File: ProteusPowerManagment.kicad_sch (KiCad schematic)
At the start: 0 parts

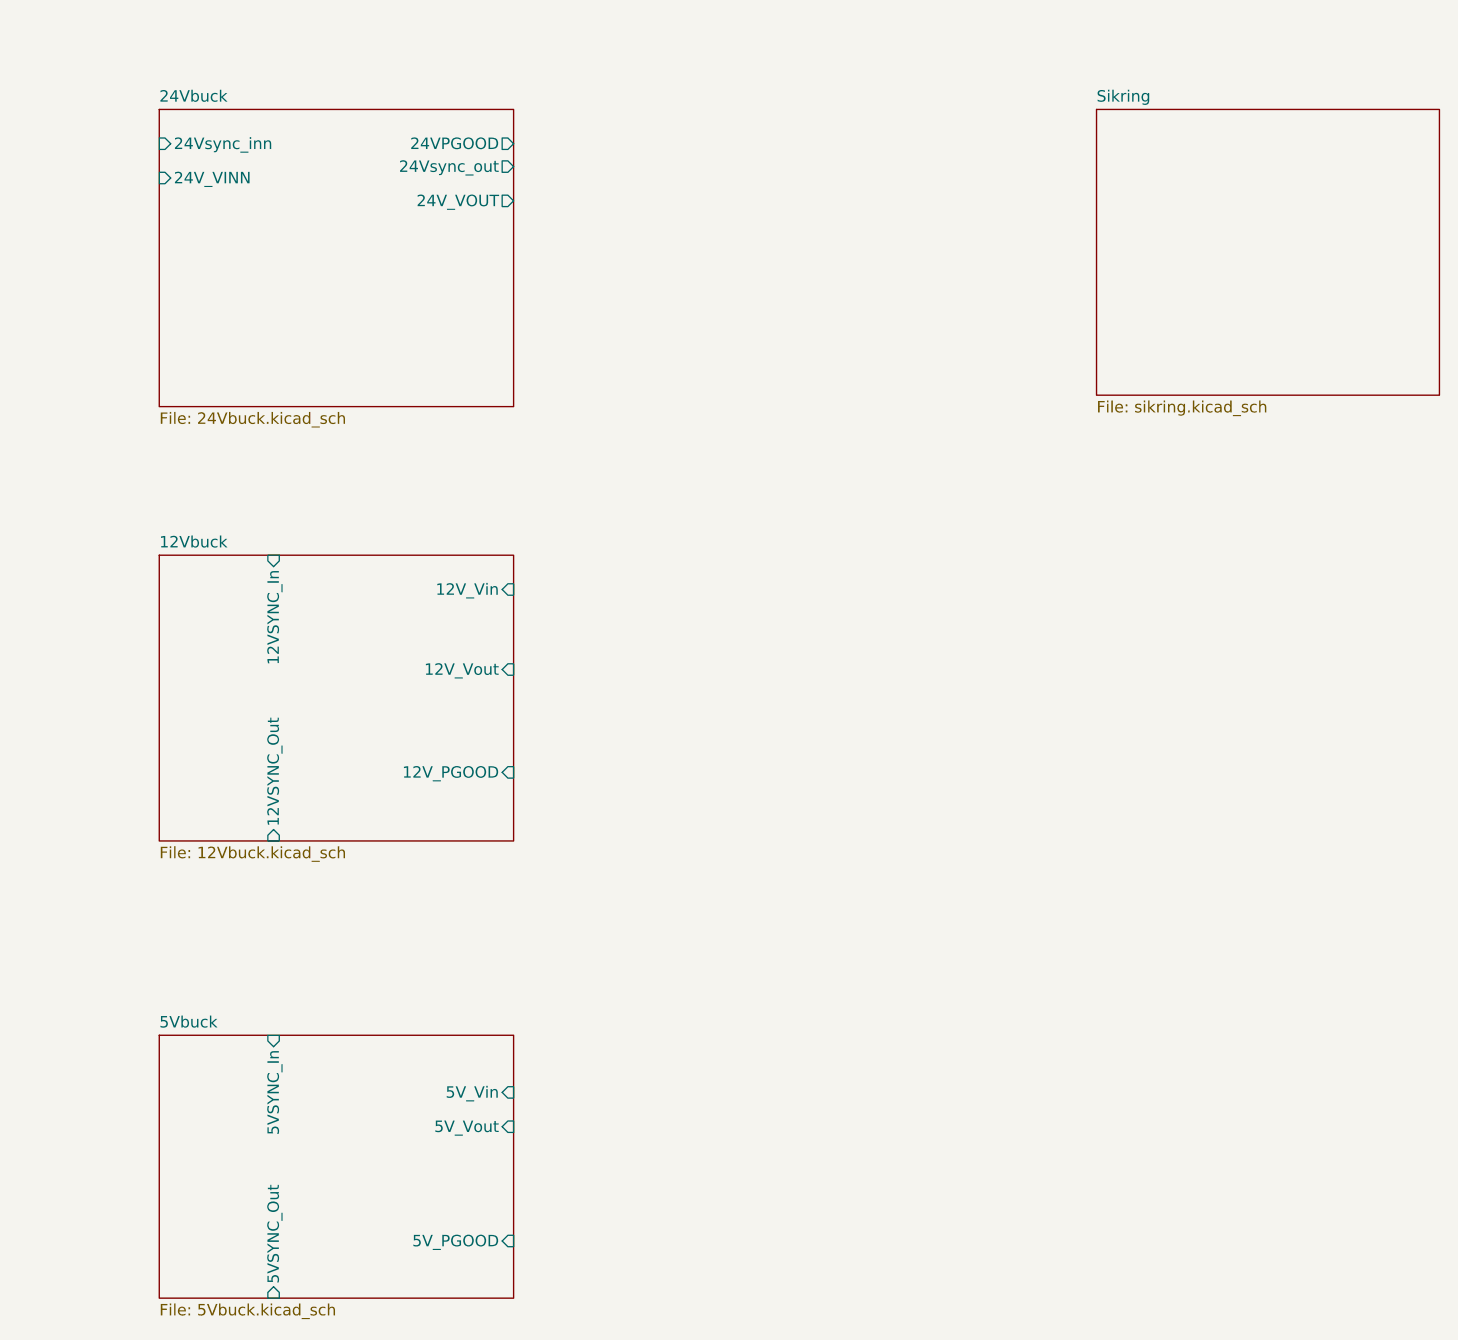
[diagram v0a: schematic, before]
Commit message: lagt inn alle ideele komp mangler å finne faktiske komponenter
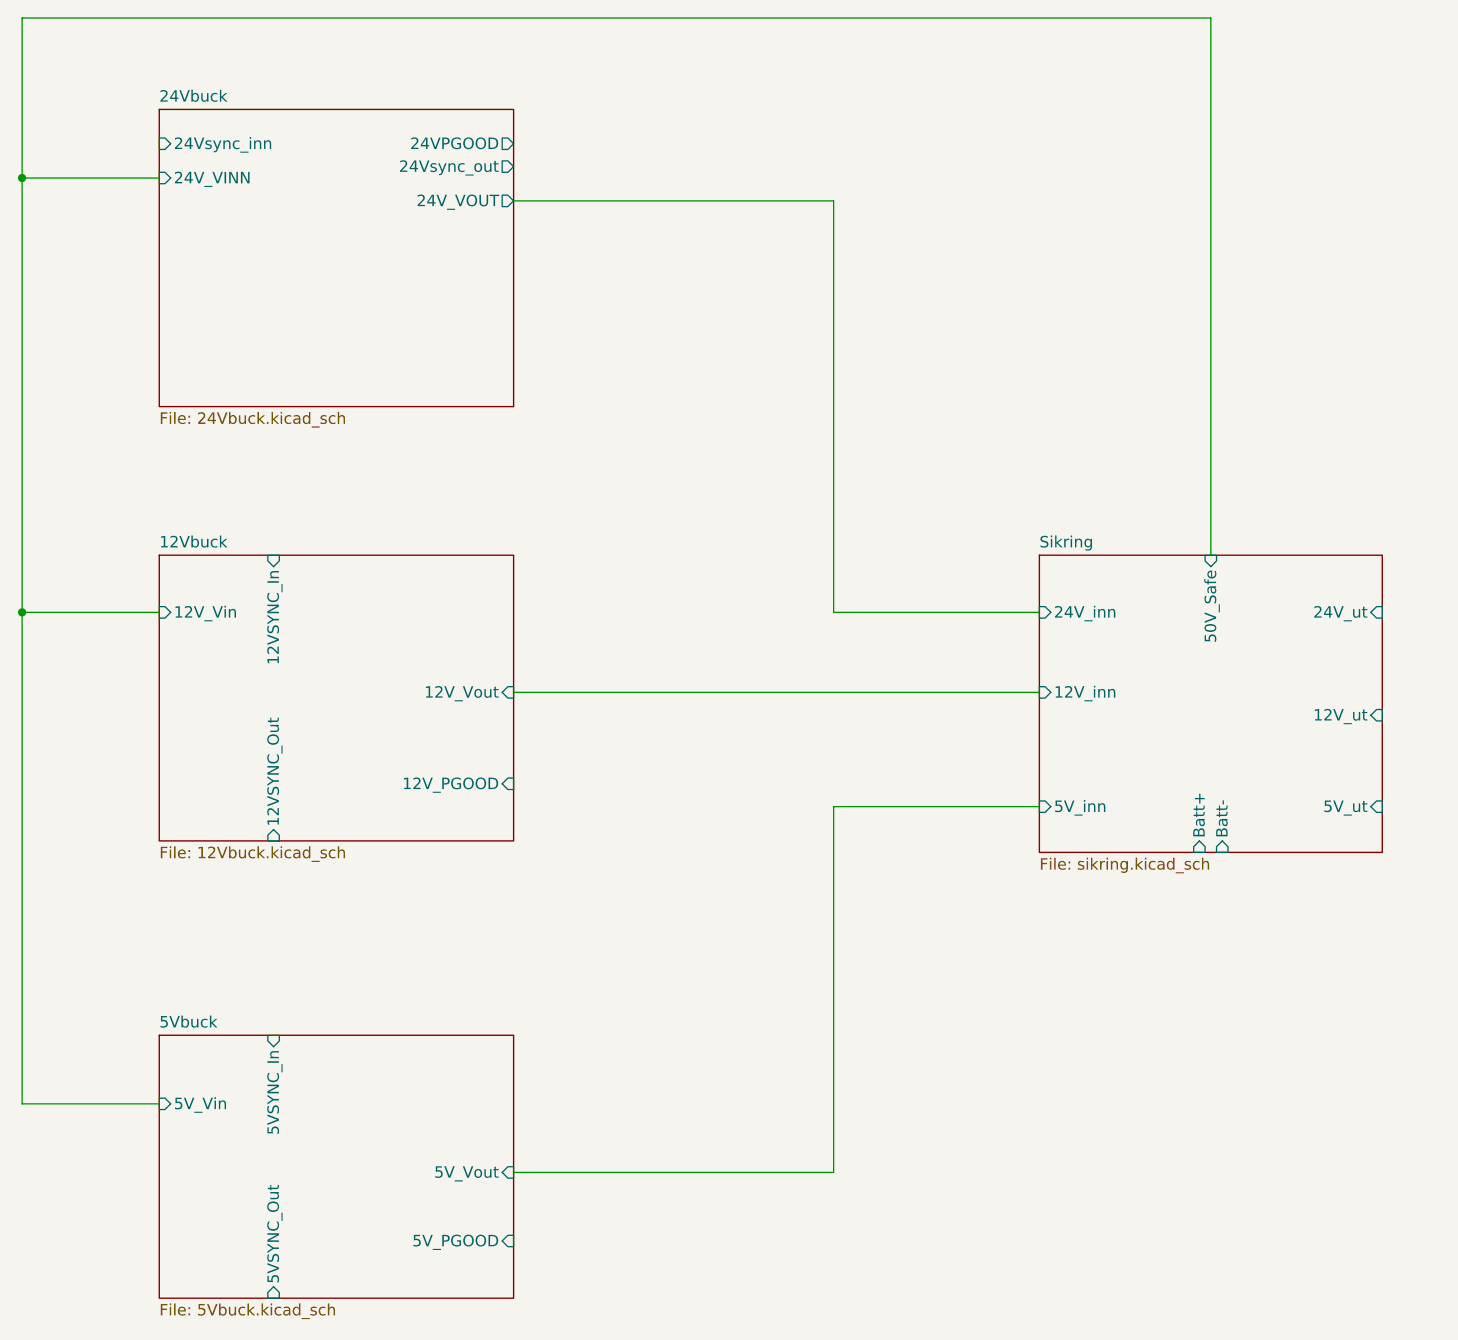
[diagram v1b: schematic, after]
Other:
- sheet Sikring ports: added 12V_inn, 12V_ut, 24V_inn, 24V_ut, 50V_Safe, 5V_inn, 5V_ut, Batt+, Batt-; removed none
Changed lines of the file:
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@@
 	(generator_version "10.0")
 	(paper "A4")
+	(junction
+		(at 24.13 95.25)
+		(diameter 0)
+		(color 0 0 0 0)
+	)
+	(junction
+		(at 24.13 46.99)
+		(diameter 0)
+		(color 0 0 0 0)
+	)
+	(wire
+		(pts
+			(xy 78.74 104.14) (xy 137.16 104.14)
+		)
+		(stroke
+			(width 0)
+			(type default)
+		)
+	)
+	(wire
+		(pts
+			(xy 24.13 46.99) (xy 39.37 46.99)
+		)
+		(stroke
+			(width 0)
+			(type default)
+		)
+	)
+	(wire
+		(pts
+			(xy 78.74 49.53) (xy 114.3 49.53)
+		)
+		(stroke
+			(width 0)
+			(type default)
+		)
+	)
+	(wire
+		(pts
+			(xy 114.3 95.25) (xy 137.16 95.25)
+		)
+		(stroke
+			(width 0)
+			(type default)
+		)
+	)
+	(wire
+		(pts
+			(xy 156.21 88.9) (xy 156.21 29.21)
+		)
+		(stroke
+			(width 0)
+			(type default)
+		)
+	)
+	(wire
+		(pts
+			(xy 114.3 49.53) (xy 114.3 95.25)
+		)
+		(stroke
+			(width 0)
+			(type default)
+		)
+	)
+	(wire
+		(pts
+			(xy 39.37 95.25) (xy 24.13 95.25)
+		)
+		(stroke
+			(width 0)
+			(type default)
+		)
+	)
+	(wire
+		(pts
+			(xy 24.13 46.99) (xy 24.13 149.86)
+		)
+		(stroke
+			(width 0)
+			(type default)
+		)
+	)
+	(wire
+		(pts
+			(xy 24.13 149.86) (xy 39.37 149.86)
+		)
+		(stroke
+			(width 0)
+			(type default)
+		)
+	)
+	(wire
+		(pts
+			(xy 24.13 29.21) (xy 24.13 46.99)
+		)
+		(stroke
+			(width 0)
+			(type default)
+		)
+	)
+	(wire
+		(pts
+			(xy 114.3 157.48) (xy 114.3 116.84)
+		)
+		(stroke
+			(width 0)
+			(type default)
+		)
+	)
+	(wire
+		(pts
+			(xy 78.74 157.48) (xy 114.3 157.48)
+		)
+		(stroke
+			(width 0)
+			(type default)
+		)
+	)
+	(wire
+		(pts
+			(xy 156.21 29.21) (xy 24.13 29.21)
+		)
+		(stroke
+			(width 0)
+			(type default)
+		)
+	)
+	(wire
+		(pts
+			(xy 114.3 116.84) (xy 137.16 116.84)
+		)
+		(stroke
+			(width 0)
+			(type default)
+		)
+	)
 	(sheet
 		(at 39.37 39.37)
@@
 	)
 	(sheet
-		(at 143.51 39.37)
-		(size 38.1 31.75)
+		(at 137.16 88.9)
+		(size 38.1 33.02)
 		(exclude_from_sim no)
 		(in_bom yes)
@@
 		)
 		(property "Sheetname" "Sikring"
-			(at 143.51 38.6584 0)
+			(at 137.16 88.1884 0)
 			(show_name no)
 			(do_not_autoplace no)
@@
 		)
 		(property "Sheetfile" "sikring.kicad_sch"
-			(at 143.51 71.7046 0)
+			(at 137.16 122.5046 0)
 			(show_name no)
 			(do_not_autoplace no)
@@
 				)
 				(justify left top)
+			)
+		)
+		(pin "5V_inn" input
+			(at 137.16 116.84 180)
+			(effects
+				(font
+					(size 1.27 1.27)
+				)
+				(justify left)
+			)
+		)
+		(pin "5V_ut" input
+			(at 175.26 116.84 0)
+			(effects
+				(font
+					(size 1.27 1.27)
+				)
+				(justify right)
+			)
+		)
+		(pin "12V_inn" input
+			(at 137.16 104.14 180)
+			(effects
+				(font
+					(size 1.27 1.27)
+				)
+				(justify left)
+			)
+		)
+		(pin "12V_ut" input
+			(at 175.26 106.68 0)
+			(effects
+				(font
+					(size 1.27 1.27)
+				)
+				(justify right)
+			)
+		)
+		(pin "24V_inn" input
+			(at 137.16 95.25 180)
+			(effects
+				(font
+					(size 1.27 1.27)
+				)
+				(justify left)
+			)
+		)
+		(pin "24V_ut" input
+			(at 175.26 95.25 0)
+			(effects
+				(font
+					(size 1.27 1.27)
+				)
+				(justify right)
+			)
+		)
+		(pin "50V_Safe" input
+			(at 156.21 88.9 90)
+			(effects
+				(font
+					(size 1.27 1.27)
+				)
+				(justify right)
+			)
+		)
+		(pin "Batt+" input
+			(at 154.94 121.92 270)
+			(effects
+				(font
+					(size 1.27 1.27)
+				)
+				(justify left)
+			)
+		)
+		(pin "Batt-" input
+			(at 157.48 121.92 270)
+			(effects
+				(font
+					(size 1.27 1.27)
+				)
+				(justify left)
 			)
 		)
@@
 		)
 		(pin "12V_PGOOD" input
-			(at 78.74 113.03 0)
+			(at 78.74 114.3 0)
 			(effects
 				(font
@@
 		)
 		(pin "12V_Vin" input
-			(at 78.74 92.71 0)
-			(effects
-				(font
-					(size 1.27 1.27)
-				)
-				(justify right)
+			(at 39.37 95.25 180)
+			(effects
+				(font
+					(size 1.27 1.27)
+				)
+				(justify left)
 			)
 		)
 		(pin "12V_Vout" input
-			(at 78.74 101.6 0)
+			(at 78.74 104.14 0)
 			(effects
 				(font
@@
 		)
 		(pin "5V_Vin" input
-			(at 78.74 148.59 0)
-			(effects
-				(font
-					(size 1.27 1.27)
-				)
-				(justify right)
+			(at 39.37 149.86 180)
+			(effects
+				(font
+					(size 1.27 1.27)
+				)
+				(justify left)
 			)
 		)
 		(pin "5V_Vout" input
-			(at 78.74 152.4 0)
-			(effects
-				(font
+			(at 78.74 157.48 0)
+			(effects
+				(font
